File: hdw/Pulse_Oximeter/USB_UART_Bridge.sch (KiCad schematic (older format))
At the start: 27 parts, among them J1201 USB_B_Mini, U1201 TLV6700, U1202 FT234XD, U1203 TPD3S014DBVR

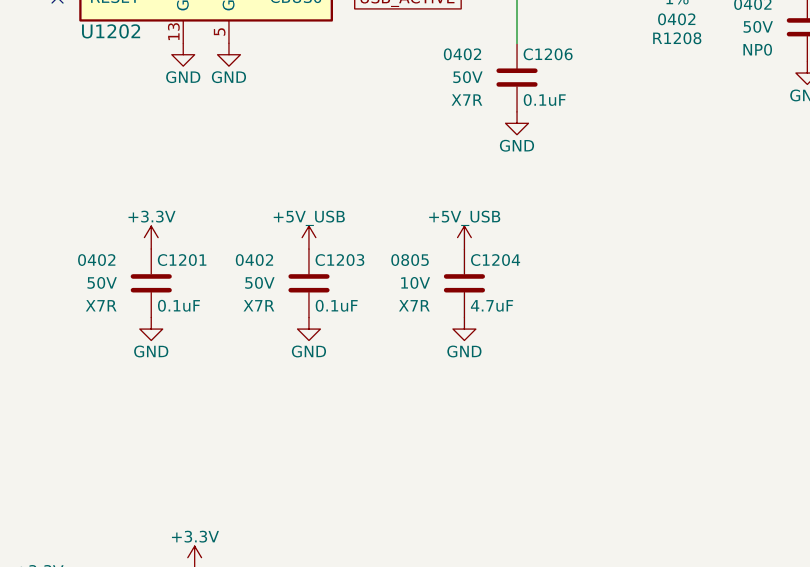
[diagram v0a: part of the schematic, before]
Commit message: More part arrangements
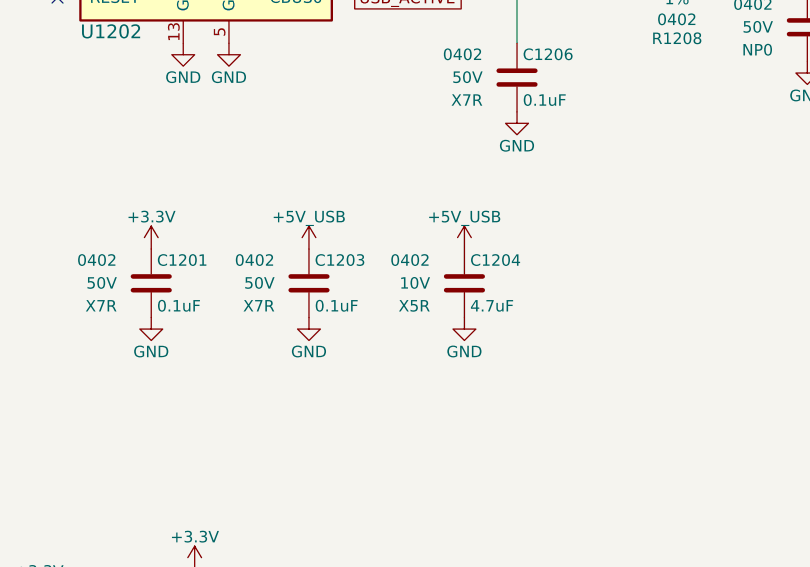
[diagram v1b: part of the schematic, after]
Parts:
- C1204: footprint Capacitors_SMD:C_0805 -> Capacitors_SMD:C_0402; Dielectric X7R -> X5R; Digi-Key PN 1276-2972-1-ND -> 490-14306-1-ND; display_footprint 0805 -> 0402
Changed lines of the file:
@@
 $Descr A 11000 8500
 encoding utf-8
-Sheet 12 23
+Sheet 12 21
 Title "Pulse Oximeter"
 Date "2019-01-03"
@@
 F 0 "C1204" H 4675 4940 50  0000 L CNN
 F 1 "4.7uF" H 4675 4740 50  0000 L CNN
-F 2 "Capacitors_SMD:C_0805" H 4688 4690 50  0001 C CNN
+F 2 "Capacitors_SMD:C_0402" H 4688 4690 50  0001 C CNN
 F 3 "" H 4675 4940 50  0001 C CNN
-F 4 "0805" H 4500 4940 50  0000 R CNN "display_footprint"
+F 4 "0402" H 4500 4940 50  0000 R CNN "display_footprint"
 F 5 "10V" H 4500 4840 50  0000 R CNN "Voltage"
-F 6 "X7R" H 4500 4740 50  0000 R CNN "Dielectric"
-F 7 "1276-2972-1-ND" H 5075 5340 60  0001 C CNN "Digi-Key PN"
+F 6 "X5R" H 4500 4740 50  0000 R CNN "Dielectric"
+F 7 "490-14306-1-ND" H 5075 5340 60  0001 C CNN "Digi-Key PN"
 	1    4650 4840
 	1    0    0    -1
